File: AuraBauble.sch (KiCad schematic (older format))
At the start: 20 parts, among them J1 USB_A, J2 SWD, Q1 Q_NMOS_DGS, SW1 RESET_SW, U1 LP5912-3.3DRV, U2 ATSAMD11D14A-U, Y1 *DNP*

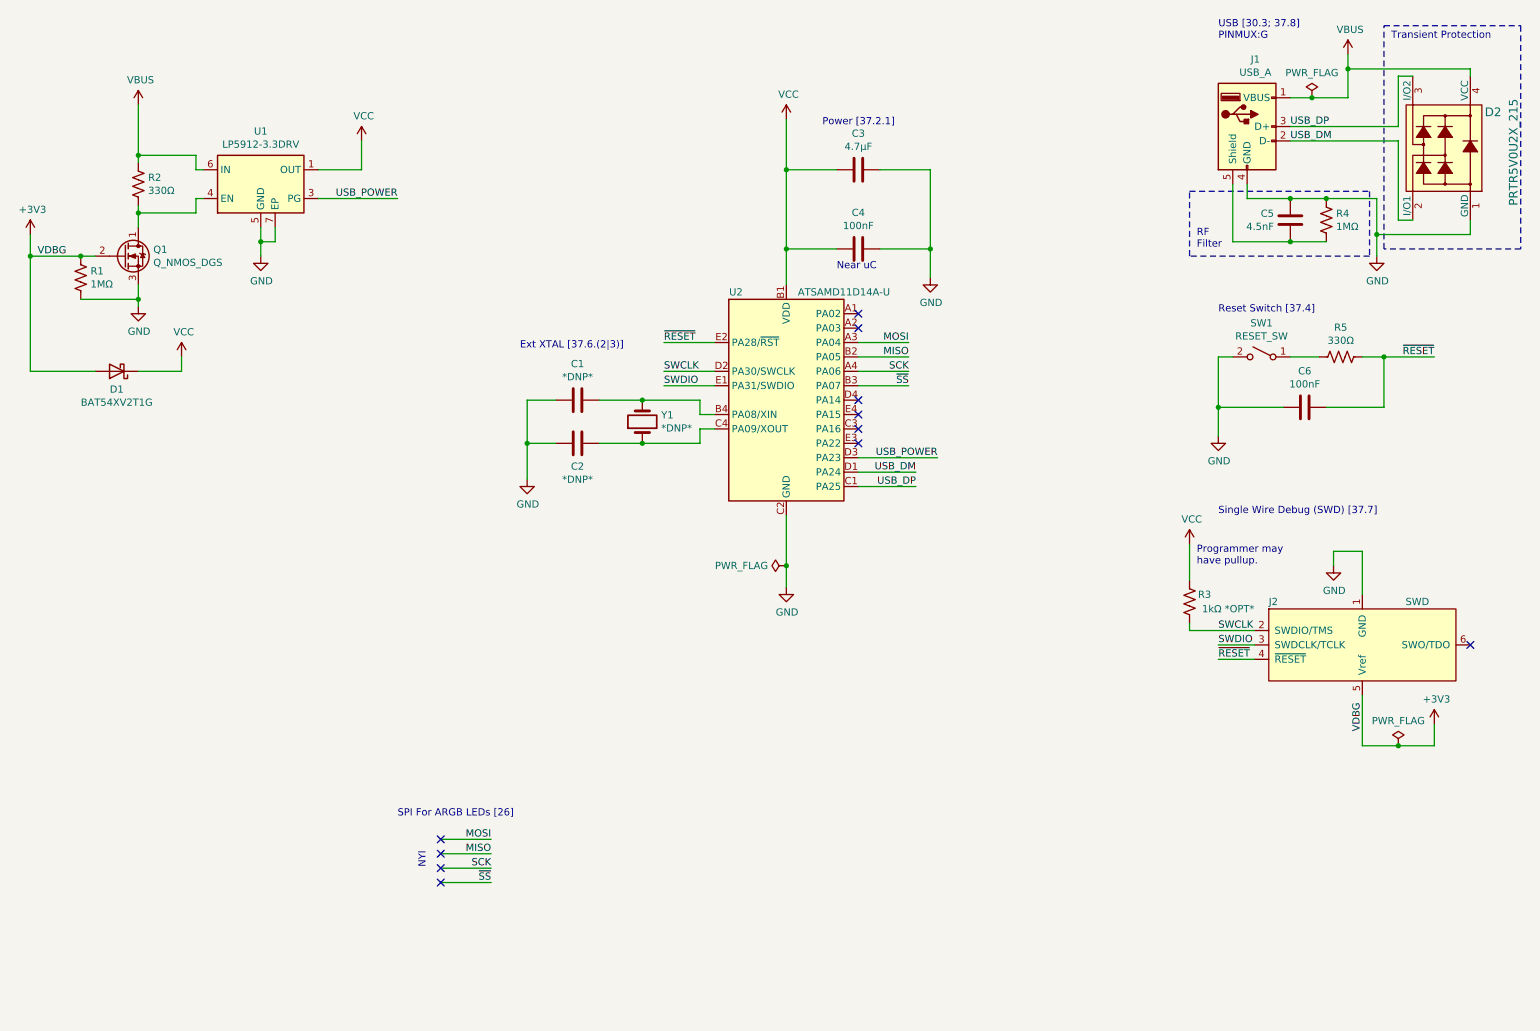
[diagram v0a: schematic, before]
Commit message: Schematic nearly r0.
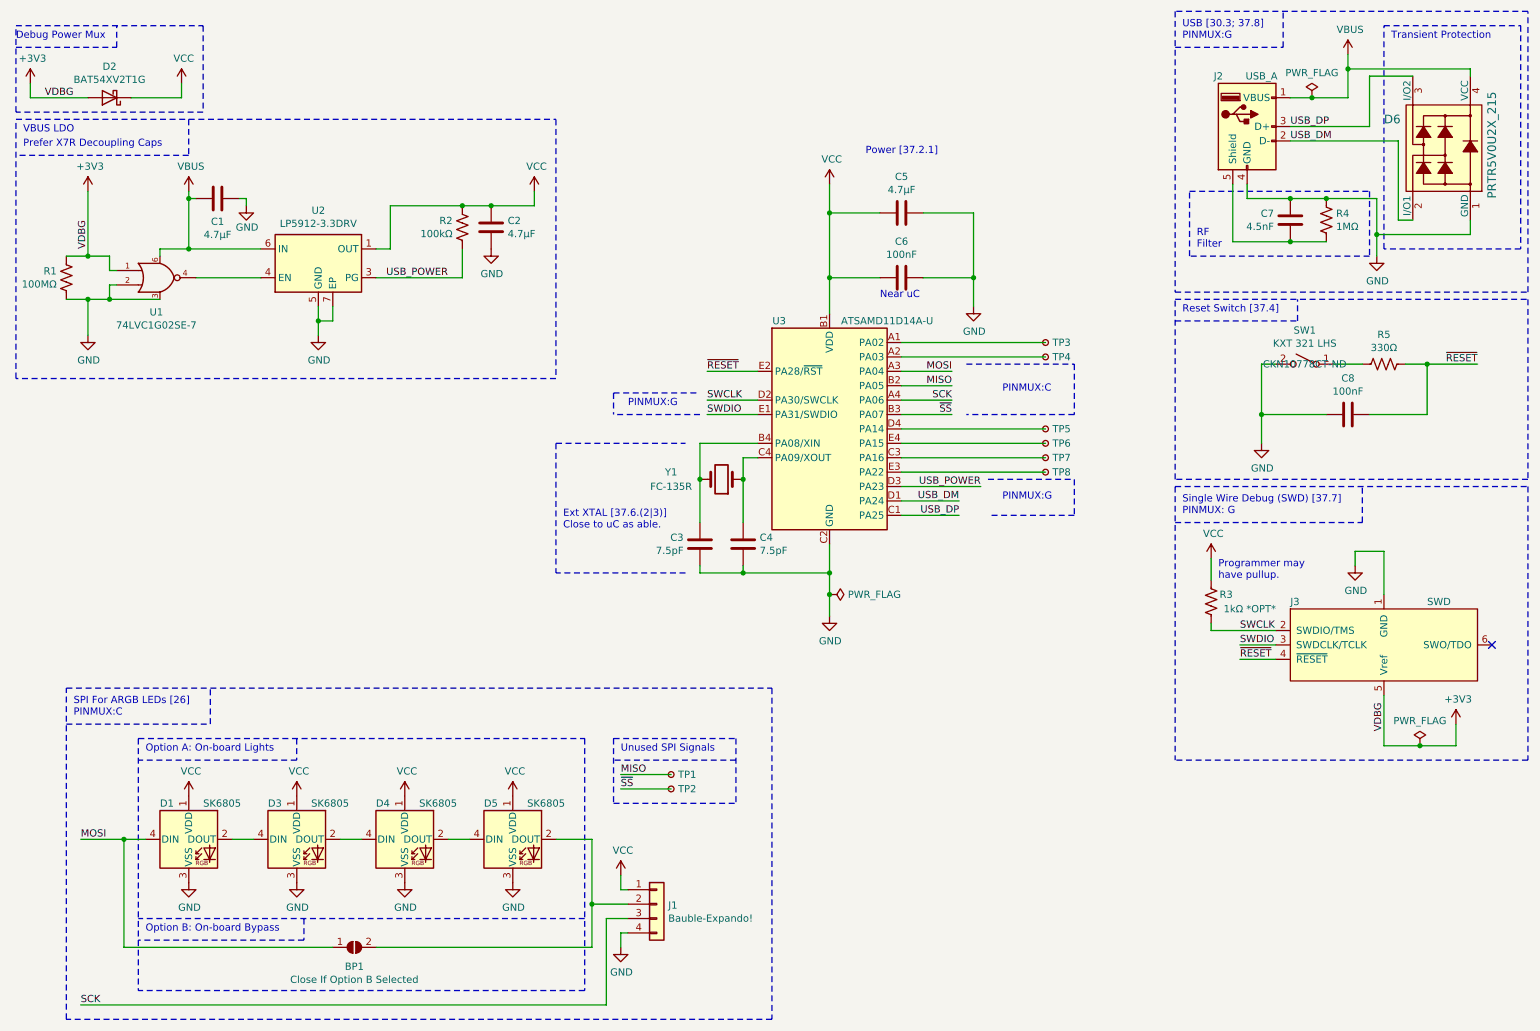
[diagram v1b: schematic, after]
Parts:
- removed Q1: Q_NMOS_DGS, symbol Device:Q_NMOS_DGS
- added BP1: Close If Option B Selected, symbol Jumper:SolderJumper_2_Open
- added C1, C2: 4.7µF, Capacitor_SMD:C_0603_1608Metric, symbol Device:C
- added D1, D3, D4, D5: SK6805, LED_SMD:LED_SK6812_EC15_1.5x1.5mm, symbol LED:WS2812B
- added J1: Bauble-Expando!, symbol Connector_Generic:Conn_01x04
- added TP1, TP2, TP3, TP4, TP5, TP6, TP7, TP8: TestPoint_Small, TestPoint:TestPoint_Pad_D1.0mm, symbol Connector:TestPoint_Small
- added U1: 74LVC1G02SE-7, Package_TO_SOT_SMD:SOT-353_SC-70-5, symbol AuraBauble_Custom:74LVC1G02
- C3: renamed from C1; value *DNP* -> 7.5pF; footprint (none) -> Capacitor_SMD:C_0603_1608Metric
- C4: renamed from C2; value *DNP* -> 7.5pF; footprint (none) -> Capacitor_SMD:C_0603_1608Metric
- C5: renamed from C3; footprint (none) -> Capacitor_SMD:C_0603_1608Metric
- C6: renamed from C4; footprint (none) -> Capacitor_SMD:C_0603_1608Metric
- C7: renamed from C5; footprint (none) -> Capacitor_SMD:C_0603_1608Metric
- C8: renamed from C6; footprint (none) -> Capacitor_SMD:C_0603_1608Metric
- D2: renamed from D1; footprint (none) -> Diode_SMD:D_SOD-523; Digi-Key (none) -> BAT54XV2T1GOSCT-ND
- J3: renamed from J2; footprint (none) -> Connector_DebugEdge:DebugEdge_2x05_Target
- R1: value 1MΩ -> 100MΩ; footprint (none) -> Resistor_SMD:R_0603_1608Metric
- R2: value 330Ω -> 100kΩ; footprint (none) -> Resistor_SMD:R_0603_1608Metric
- R3, R4, R5: footprint (none) -> Resistor_SMD:R_0603_1608Metric
- SW1: value RESET_SW -> KXT 321 LHS; footprint (none) -> Button_Switch_SMD:SW_SPST_CK_KXT3; Digi-Key (none) -> CKN10778CT-ND
- U2: renamed from U1; Digi-Key (none) -> 296-44153-1-ND
- Y1: value *DNP* -> FC-135R; footprint (none) -> Crystal:Crystal_SMD_3215-2Pin_3.2x1.5mm; Digi-Key (none) -> FC-135 32.7680KA-AG5
- renumbered D2 to D6, J1 to J2, U2 to U3
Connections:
- net +3V3: now also U1.1
- net GND: now also C1.2, C2.1, D1.3 (VSS), D3.3 (VSS), D4.3 (VSS), D5.3 (VSS), J1.4 (Pin_4), U1.2, U1.3 (GND)
- net MISO: now also TP1.1
- net MOSI: now also BP1.1 (A), D1.4 (DIN)
- net SCK: now also J1.3 (Pin_3)
- net USB_POWER: now also R2.2
- net VBUS: now also C1.1, U1.6 (VCC); no longer R2.2
- net VCC: now also R2.1, C2.2, D1.1 (VDD), D3.1 (VDD), D4.1 (VDD), D5.1 (VDD), J1.1 (Pin_1)
- net ~SS~: now also TP2.1
- net at U3.A1 (PA02): now also TP3.1
- net at U3.A2 (PA03): now also TP4.1
- net at U3.C3 (PA16): now also TP7.1
- net at U3.D4 (PA14): now also TP5.1
- net at U3.E3 (PA22): now also TP8.1
- net at U3.E4 (PA15): now also TP6.1
- net at U2.4 (EN): now also U1.4; no longer R2.1
- new net: D1.2 (DOUT), D3.4 (DIN)
- new net: D3.2 (DOUT), D4.4 (DIN)
- new net: D4.2 (DOUT), D5.4 (DIN)
- new net: BP1.2 (B), D5.2 (DOUT), J1.2 (Pin_2)
- no-connect marks 11 -> 1
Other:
- note added: "Debug Power Mux"
- note added: "Ext XTAL [37.6.(2|3)]\nClose to uC as able."
- note added: "Option A: On-board Lights"
- note added: "Option B: On-board Bypass"
- note added: "PINMUX:C"
- note added: "PINMUX:G"
- note added: "Prefer X7R Decoupling Caps"
- note added: "SPI For ARGB LEDs [26]\nPINMUX:C"
- note added: "Single Wire Debug (SWD) [37.7]\nPINMUX: G"
- note added: "Unused SPI Signals"
- note added: "VBUS LDO"
- note removed: "Ext XTAL [37.6.(2|3)]"
- note removed: "NYI"
- note removed: "SPI For ARGB LEDs [26]"
- note removed: "Single Wire Debug (SWD) [37.7]"
- moved on the sheet: C3, C4, C5, C6, C8, D2, J3, R1, R3, R5, SW1, U2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
